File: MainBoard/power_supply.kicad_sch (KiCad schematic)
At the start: 7 parts, among them P1 USB_C_Receptacle_USB2.0_14P, U1 MCP73811T-420I-OT

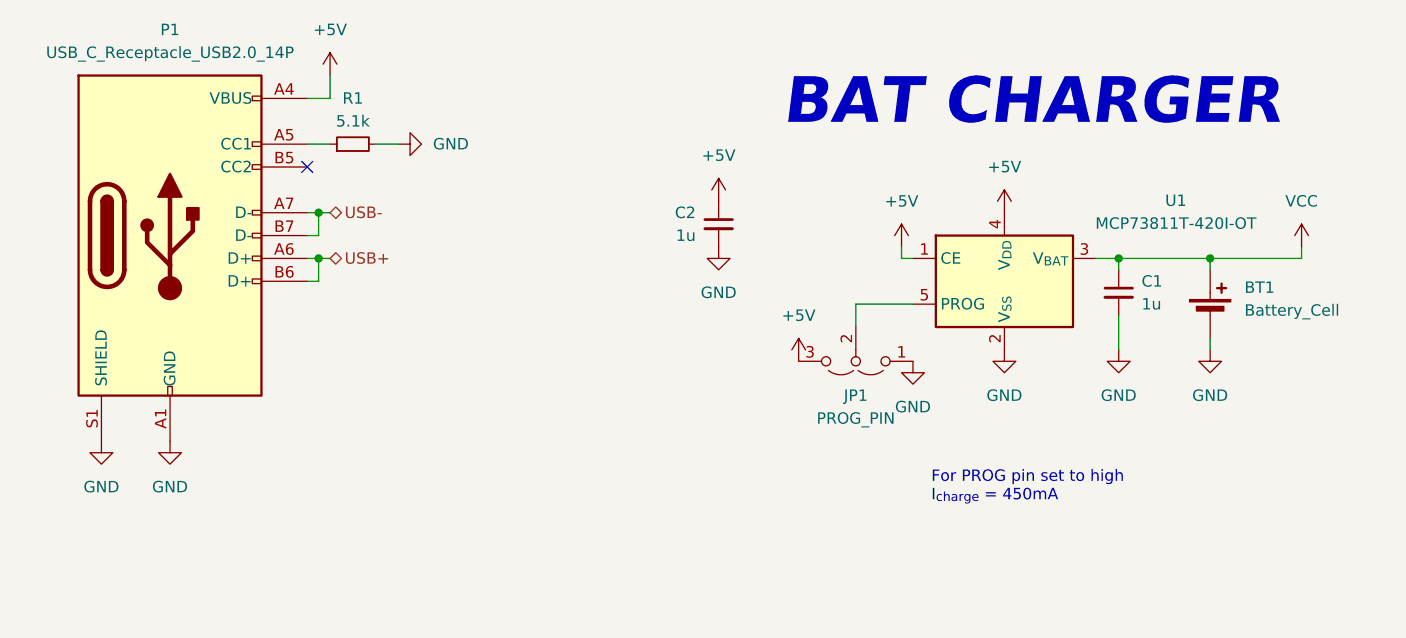
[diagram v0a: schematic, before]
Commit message: change schematic
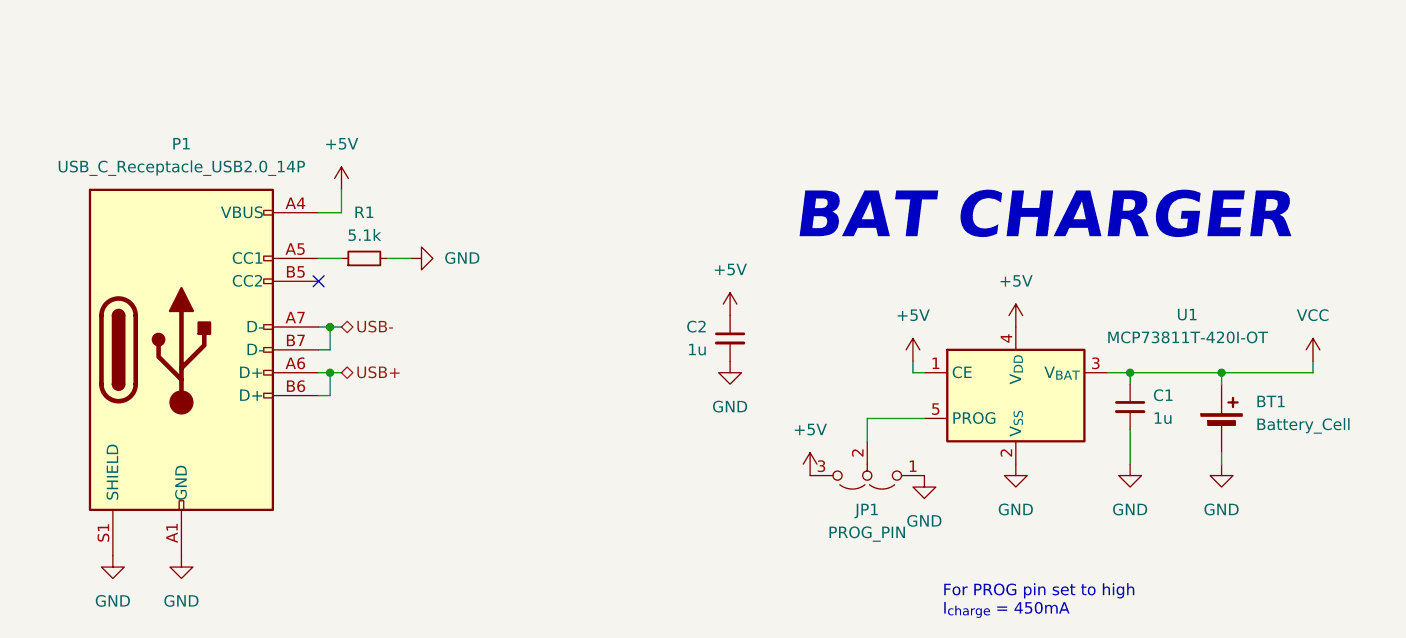
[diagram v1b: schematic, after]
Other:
- moved on the sheet: BT1, C1, C2, JP1, P1, R1, U1

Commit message: Udpate project variables and add texts
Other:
- title: blob -> VirtualBlob
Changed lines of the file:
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@@
 	(paper "A4")
 	(title_block
-		(title "blob")
+		(title "VirtualBlob")
 		(date "2025-09-15")
 		(rev "0.4.0")

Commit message: Change naming of project
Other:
- company: Miłosz Derżko -> ${Company}
- title: VirtualBlob -> ${ProjectTitle}
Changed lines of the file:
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@@
 	(paper "A4")
 	(title_block
-		(title "VirtualBlob")
+		(title "${ProjectTitle}")
 		(date "2025-09-15")
-		(rev "0.4.0")
-		(company "Miłosz Derżko")
+		(rev "${Revision}")
+		(company "${Company}")
 	)
 	(text "BAT CHARGER"
@@
 		)
 		(instances
-			(project "mainboard"
+			(project "MainBoard"
 				(path "/9e709b97-b403-4027-b7d8-a3ed3b3557e2/84d390ca-b239-4386-b2d6-b74c29a08765"
 					(reference "#PWR0104")
@@
 		)
 		(instances
-			(project "mainboard"
+			(project "MainBoard"
 				(path "/9e709b97-b403-4027-b7d8-a3ed3b3557e2/84d390ca-b239-4386-b2d6-b74c29a08765"
 					(reference "#PWR021")
@@
 		)
 		(instances
-			(project "mainboard"
+			(project "MainBoard"
 				(path "/9e709b97-b403-4027-b7d8-a3ed3b3557e2/84d390ca-b239-4386-b2d6-b74c29a08765"
 					(reference "#PWR014")
@@
 		)
 		(instances
-			(project "mainboard"
+			(project "MainBoard"
 				(path "/9e709b97-b403-4027-b7d8-a3ed3b3557e2/84d390ca-b239-4386-b2d6-b74c29a08765"
 					(reference "C2")
@@
 		)
 		(instances
-			(project "mainboard"
+			(project "MainBoard"
 				(path "/9e709b97-b403-4027-b7d8-a3ed3b3557e2/84d390ca-b239-4386-b2d6-b74c29a08765"
 					(reference "#PWR012")
@@
 		)
 		(instances
-			(project "mainboard"
+			(project "MainBoard"
 				(path "/9e709b97-b403-4027-b7d8-a3ed3b3557e2/84d390ca-b239-4386-b2d6-b74c29a08765"
 					(reference "U1")
@@
 		)
 		(instances
-			(project "mainboard"
+			(project "MainBoard"
 				(path "/9e709b97-b403-4027-b7d8-a3ed3b3557e2/84d390ca-b239-4386-b2d6-b74c29a08765"
 					(reference "C1")
@@
 		)
 		(instances
-			(project "mainboard"
+			(project "MainBoard"
 				(path "/9e709b97-b403-4027-b7d8-a3ed3b3557e2/84d390ca-b239-4386-b2d6-b74c29a08765"
 					(reference "#PWR02")
@@
 		)
 		(instances
-			(project "mainboard"
+			(project "MainBoard"
 				(path "/9e709b97-b403-4027-b7d8-a3ed3b3557e2/84d390ca-b239-4386-b2d6-b74c29a08765"
 					(reference "#PWR0103")
@@
 		)
 		(instances
-			(project "mainboard"
+			(project "MainBoard"
 				(path "/9e709b97-b403-4027-b7d8-a3ed3b3557e2/84d390ca-b239-4386-b2d6-b74c29a08765"
 					(reference "#PWR020")
@@
 		)
 		(instances
-			(project "mainboard"
+			(project "MainBoard"
 				(path "/9e709b97-b403-4027-b7d8-a3ed3b3557e2/84d390ca-b239-4386-b2d6-b74c29a08765"
 					(reference "#PWR011")
@@
 		)
 		(instances
-			(project "mainboard"
+			(project "MainBoard"
 				(path "/9e709b97-b403-4027-b7d8-a3ed3b3557e2/84d390ca-b239-4386-b2d6-b74c29a08765"
 					(reference "#PWR04")
@@
 		)
 		(instances
-			(project "mainboard"
+			(project "MainBoard"
 				(path "/9e709b97-b403-4027-b7d8-a3ed3b3557e2/84d390ca-b239-4386-b2d6-b74c29a08765"
 					(reference "#PWR0101")
@@
 		)
 		(instances
-			(project "mainboard"
+			(project "MainBoard"
 				(path "/9e709b97-b403-4027-b7d8-a3ed3b3557e2/84d390ca-b239-4386-b2d6-b74c29a08765"
 					(reference "#PWR017")
@@
 		)
 		(instances
-			(project "mainboard"
+			(project "MainBoard"
 				(path "/9e709b97-b403-4027-b7d8-a3ed3b3557e2/84d390ca-b239-4386-b2d6-b74c29a08765"
 					(reference "#PWR016")
@@
 		)
 		(instances
-			(project "mainboard"
+			(project "MainBoard"
 				(path "/9e709b97-b403-4027-b7d8-a3ed3b3557e2/84d390ca-b239-4386-b2d6-b74c29a08765"
 					(reference "#PWR0102")
@@
 		)
 		(instances
-			(project "mainboard"
+			(project "MainBoard"
 				(path "/9e709b97-b403-4027-b7d8-a3ed3b3557e2/84d390ca-b239-4386-b2d6-b74c29a08765"
 					(reference "R1")
@@
 		)
 		(instances
-			(project "mainboard"
+			(project "MainBoard"
 				(path "/9e709b97-b403-4027-b7d8-a3ed3b3557e2/84d390ca-b239-4386-b2d6-b74c29a08765"
 					(reference "JP1")
@@
 		)
 		(instances
-			(project "mainboard"
+			(project "MainBoard"
 				(path "/9e709b97-b403-4027-b7d8-a3ed3b3557e2/84d390ca-b239-4386-b2d6-b74c29a08765"
 					(reference "BT1")
@@
 		)
 		(instances
-			(project "mainboard"
+			(project "MainBoard"
 				(path "/9e709b97-b403-4027-b7d8-a3ed3b3557e2/84d390ca-b239-4386-b2d6-b74c29a08765"
 					(reference "#PWR015")
@@
 		)
 		(instances
-			(project "mainboard"
+			(project "MainBoard"
 				(path "/9e709b97-b403-4027-b7d8-a3ed3b3557e2/84d390ca-b239-4386-b2d6-b74c29a08765"
 					(reference "P1")
